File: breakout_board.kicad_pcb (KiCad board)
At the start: 2 copper layers, 33.9 x 33.4 mm, 31 parts, among them J1 Dummy Pins, J2 Debugger, J3 USB_C_Receptacle_USB2.0_16P, U1 STM32F103C8Tx

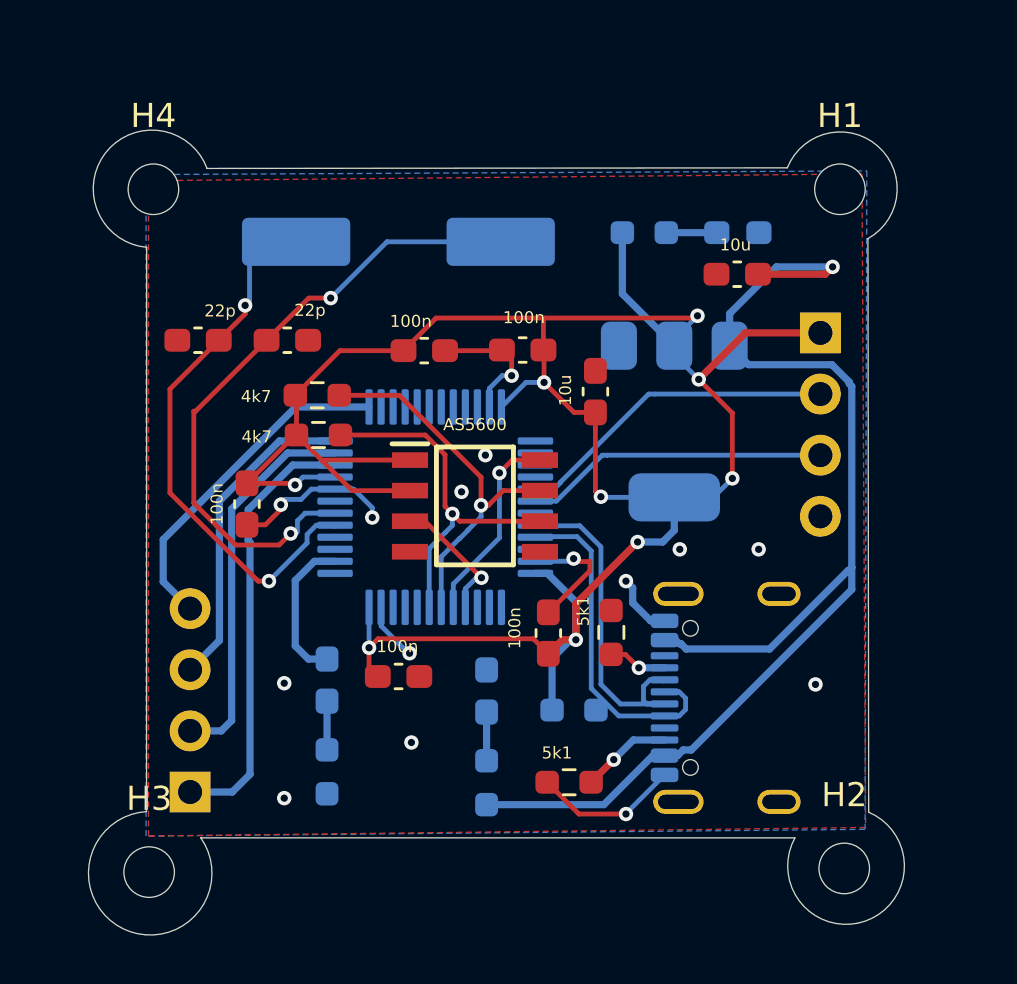
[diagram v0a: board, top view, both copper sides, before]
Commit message: Bunny ears
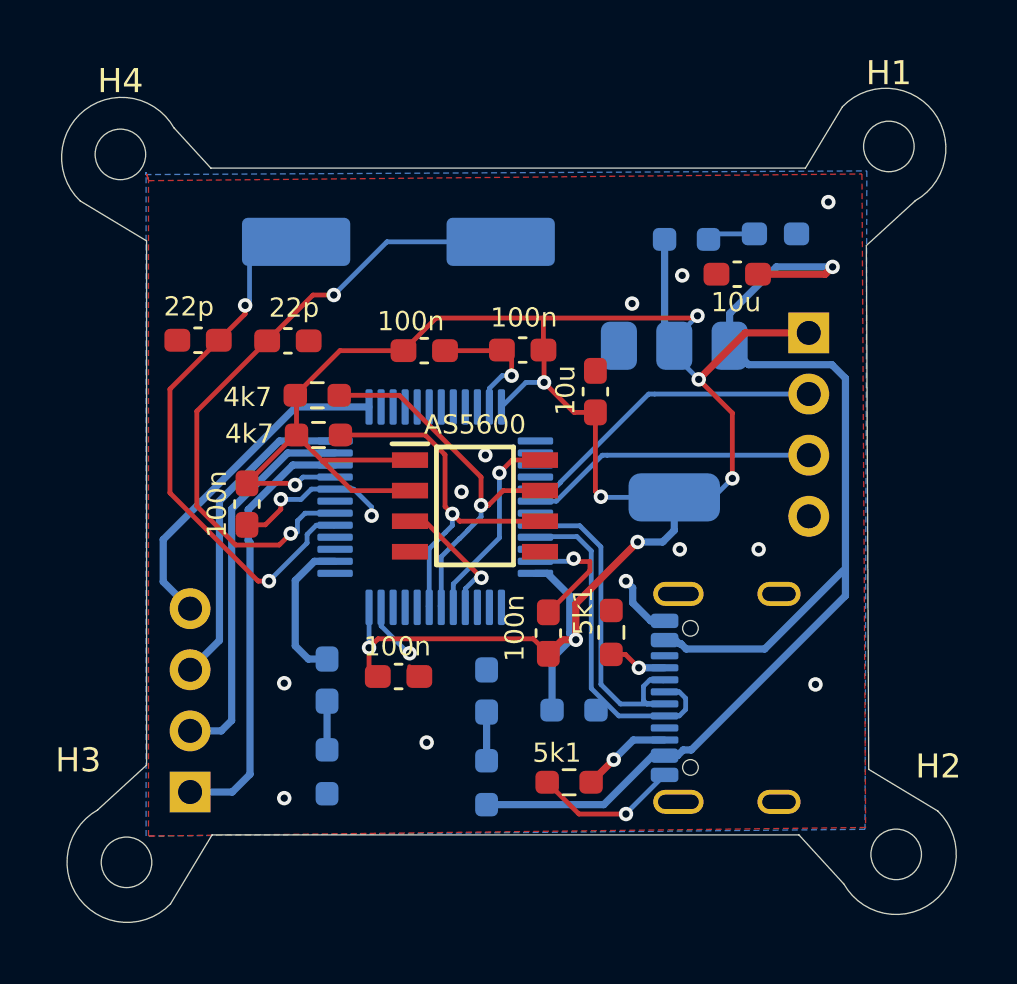
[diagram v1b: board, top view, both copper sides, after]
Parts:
- moved H1 2.70 mm to (150.4, 64.2)
- moved H2 2.24 mm to (150.7, 93.6)
- moved H4 1.99 mm to (118.4, 64.6)
- moved 1k 1.78 mm to (142.0, 68.1)
- moved LED 1.56 mm to (145.7, 67.9)
- moved H3 1.02 mm to (118.7, 94.0)
- moved J2 0.48 mm to (147.0, 72.0)
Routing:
- net VDD_c: track 100.4 -> 99.3 mm
- net GND: track 29.5 -> 30.2 mm, vias 15 -> 18
- net VBUS: track 52.1 -> 51.5 mm
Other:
- board size 33.9 x 33.4 mm -> 37.2 x 34.7 mm
